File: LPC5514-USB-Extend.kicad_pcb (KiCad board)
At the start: 2 copper layers, 55 parts, among them J1 USB_C_Receptacle_USB2.0, J2 Conn_02x05_Odd_Even, J3 Conn_02x08_Counter_Clockwise, J4 Conn_01x04, J5 Conn_02x05_Odd_Even, J6 Screw_Terminal_01x03, J7 Conn_02x10_Odd_Even, U1 LPC5514JBD64E, U2 AP1117-33, U3 TJA1042T-3, Y1 16MHz, Y2 32.768KHz

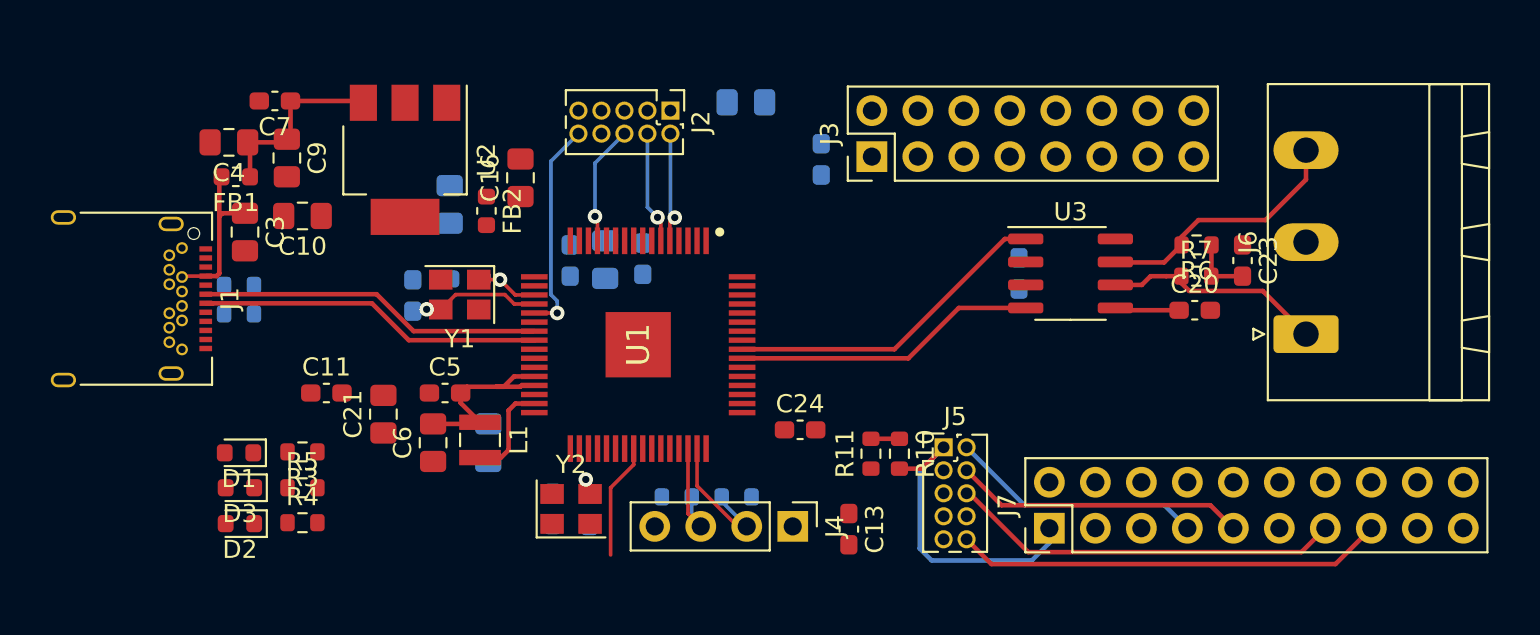
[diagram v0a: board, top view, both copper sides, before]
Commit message: update design
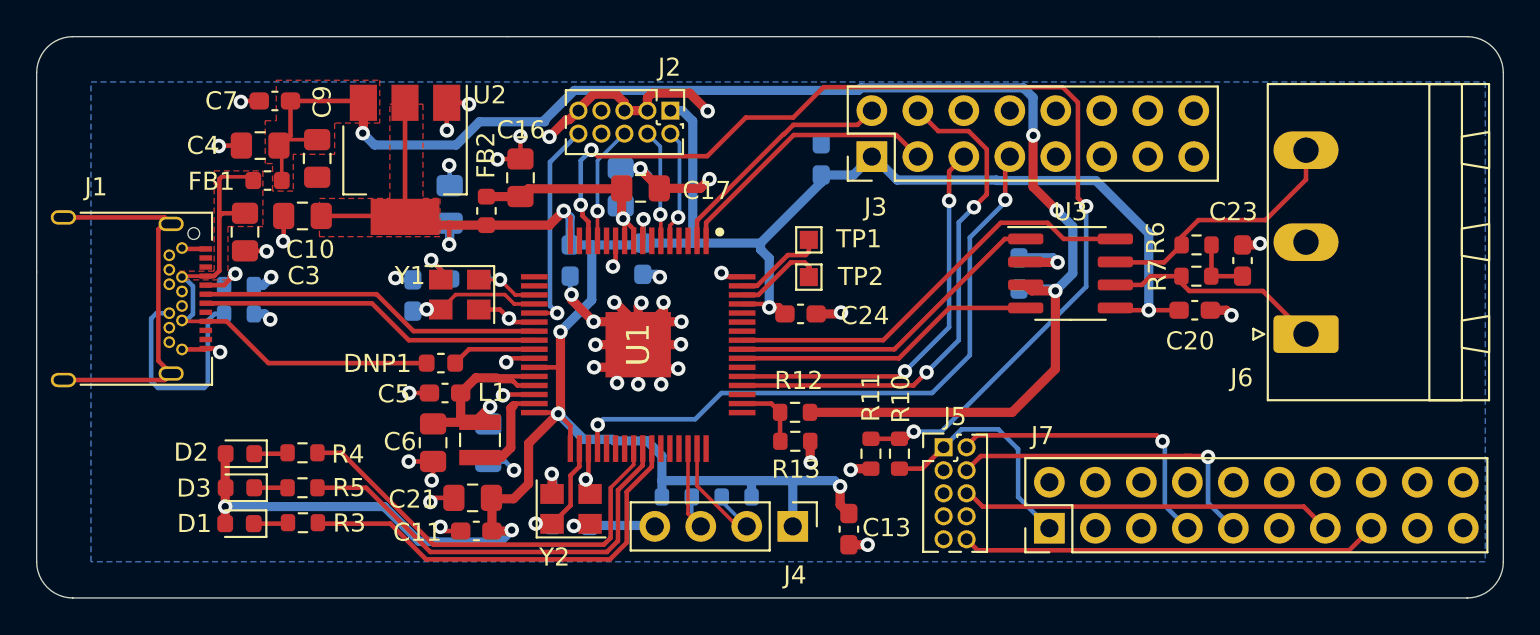
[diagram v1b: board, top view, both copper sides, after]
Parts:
- added DNP1: Ferrite_Bead_Small, Inductor_SMD:L_0603_1608Metric, F.Cu at (114.3, 105.0)
- added R12: 10K, Resistor_SMD:R_0603_1608Metric, F.Cu at (133.9, 107.7)
- added R13: 20K, Resistor_SMD:R_0603_1608Metric, F.Cu at (133.9, 109.3)
- added TP1: TestPoint, TestPoint:TestPoint_Pad_1.0x1.0mm, F.Cu at (134.6, 98.2)
- added TP2: TestPoint, TestPoint:TestPoint_Pad_1.0x1.0mm, F.Cu at (134.6, 100.3)
- C17: moved to F.Cu
- moved C11 11.3 mm to (116.3, 114.3), turned to 180 degrees
- moved C17 7.51 mm to (125.3, 95.4)
- moved C21 6.76 mm to (116.1, 112.5), turned to 180 degrees
- moved C24 6.40 mm to (134.2, 102.3)
- moved C18 4.10 mm to (124.3, 95.3), turned to 90 degrees
- moved D1 3.91 mm to (103.2, 113.9)
- moved R3 3.91 mm to (106.7, 113.8)
- moved D2 3.86 mm to (103.2, 110.0)
- moved R4 3.86 mm to (106.7, 110.0), turned to 180 degrees
- moved FB1 1.76 mm to (104.7, 94.9)
- moved C4 1.74 mm to (104.3, 93.0)
- moved C9 1.68 mm to (107.5, 93.7)
- turned R5 to 180 degrees
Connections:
- D3 pad 2: Net-(D3-Pad2) -> +3V3
- J3 pad 2: /FC3_RTS_SCL_SSEL1 -> /FC3_CTS_SDA_SSEL0
- J3 pad 3: /FC3_CTS_SDA_SSEL0 -> /FC3_RTS_SCL_SSEL1
- U1 pad 57: Net-(U1-Pad57) -> /CAN_STB
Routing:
- net +3V3: track 3.57 -> 157.2 mm, vias 0 -> 10
- net GND: track 0.00 -> 111.4 mm, vias 0 -> 52
- net +5V: track 10.5 -> 86.0 mm, vias 0 -> 4
- net /TARGET_VCC_DIV: track 1.57 -> 60.6 mm, vias 0 -> 4
- net /FC3_SCK: track 0.00 -> 35.3 mm, vias 0 -> 2
- net /FC3_TXD_SCL_MISO: track 0.00 -> 28.9 mm, vias 0 -> 2
- net /LED_R: track 0.00 -> 24.0 mm
- net /LED_B: track 0.00 -> 24.0 mm
- net /CAN_STB: track 0.00 -> 23.7 mm
- net /FC3_RXD_SDA_MOSI: track 0.00 -> 22.3 mm, vias 0 -> 2
- net Net-(J1-PadS1): track 0.00 -> 21.3 mm
- net +5VA: track 9.01 -> 28.4 mm
- net /LED_G: track 6.40 -> 23.9 mm
- net /FC3_RTS_SCL_SSEL1: track 0.00 -> 15.2 mm
- net /FC3_CTS_SDA_SSEL0: track 0.00 -> 13.3 mm
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- added copper zone on F.Cu, net +3V3
- added copper zone on F.Cu, net +5V
- added copper zone on F.Cu, net +5VA
- added copper zone on B.Cu, net GND
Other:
- board outline added: 81 x 31 mm
